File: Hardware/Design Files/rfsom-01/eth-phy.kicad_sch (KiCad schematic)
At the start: 1 part, among them U6 KSZ9131RNXI-TR

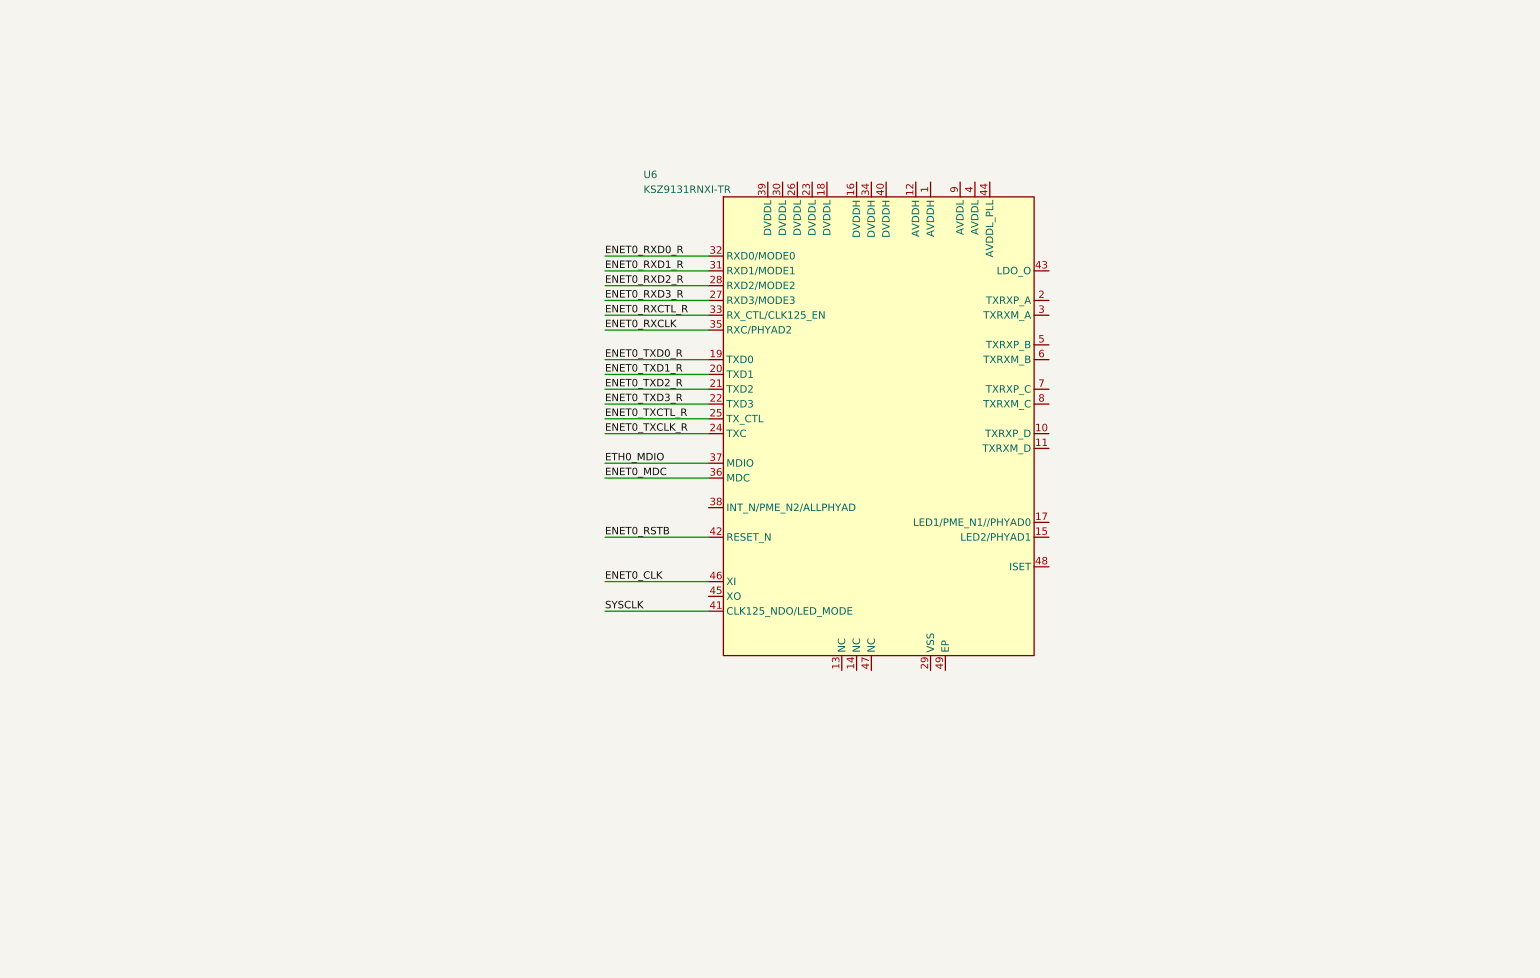
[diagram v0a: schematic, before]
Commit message: ps progress; added ftdi; mezz pinout pedinging;
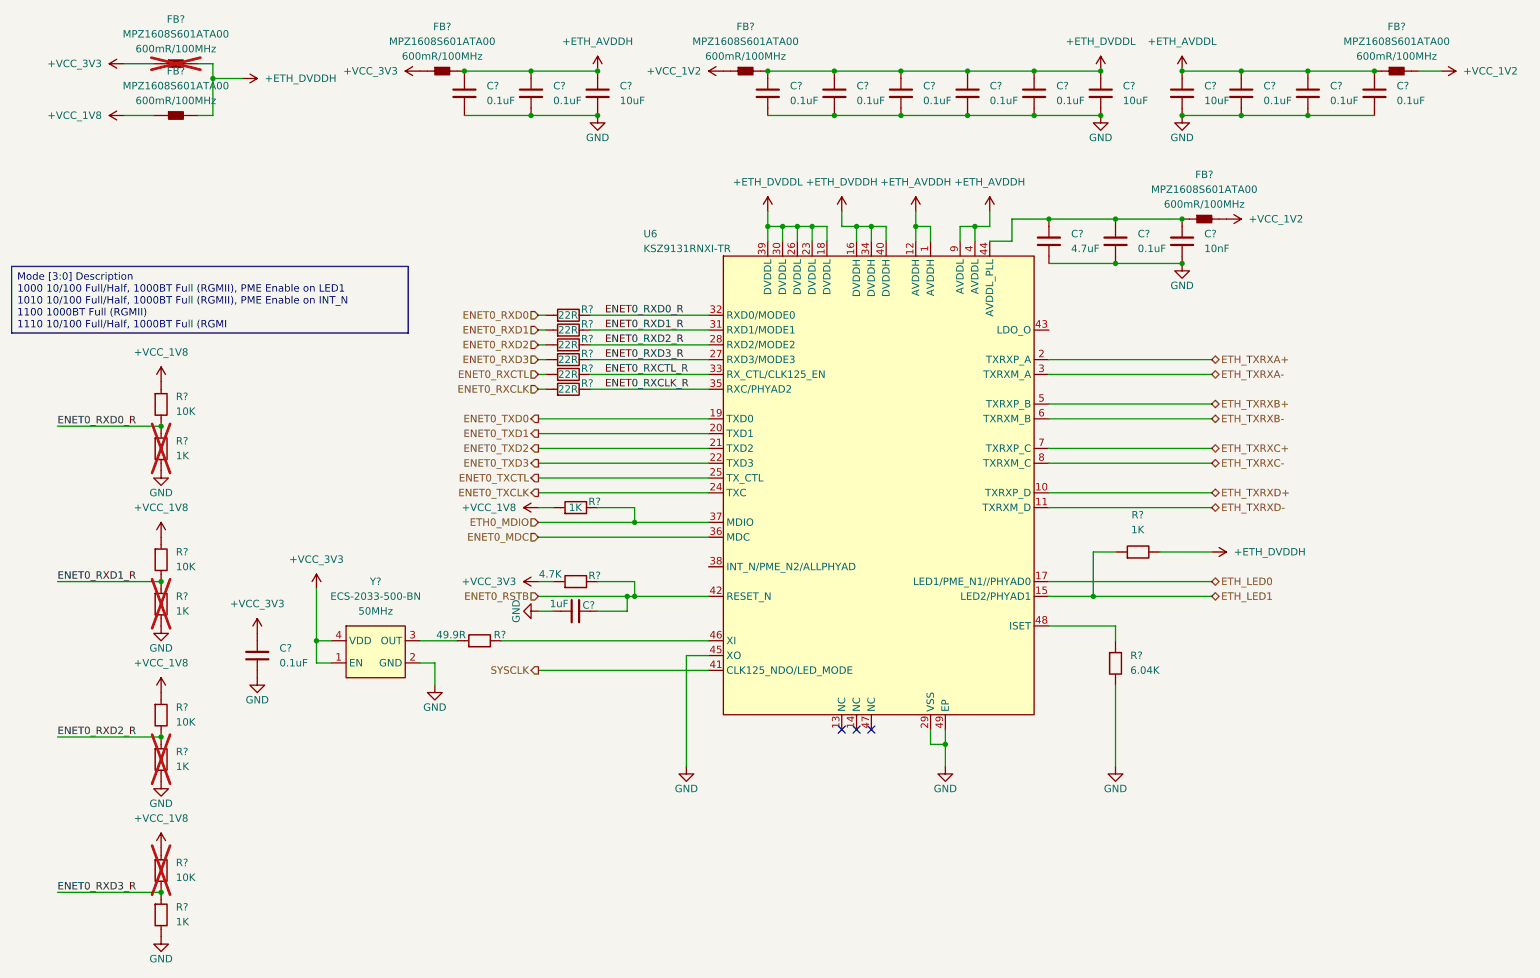
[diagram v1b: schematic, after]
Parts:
- added C? (x12): CL05B104KA5NNNC, Capacitor_SMD:C_0402_1005Metric_Pad0.74x0.62mm_HandSolder, symbol Capacitors:CL05B104KA5NNNC
- added C? (x3): CL31A106KBHNNNE, Capacitor_SMD:C_1206_3216Metric_Pad1.33x1.80mm_HandSolder, symbol Capacitors:CL31A106KBHNNNE
- added C?: CL10B105KA8NNNC, Capacitor_SMD:C_0603_1608Metric_Pad1.08x0.95mm_HandSolder, symbol Capacitors:CL10B105KA8NNNC
- added C?: CL05B103KB5NNNC, Capacitor_SMD:C_0402_1005Metric, symbol Capacitors:CL05B103KB5NNNC
- added C?: CL21B475KAFNNNE, Capacitor_SMD:C_0805_2012Metric_Pad1.18x1.45mm_HandSolder, symbol Capacitors:CL21B475KAFNNNE
- added FB? (x6): MPZ1608S601ATA00, Resistor_SMD:R_0603_1608Metric, symbol Inductors:MPZ1608S601ATA00
- added R? (x6): RC0402FR-0722RL, Resistor_SMD:R_0402_1005Metric, symbol Resistors:RC0402FR-0722RL
- added R? (x6): RC0603FR-071KL, Resistor_SMD:R_0603_1608Metric_Pad0.98x0.95mm_HandSolder, symbol Resistors:RC0603FR-071KL
- added R? (x4): RC0603FR-0710KL, Resistor_SMD:R_0603_1608Metric_Pad0.98x0.95mm_HandSolder, symbol Resistors:RC0603FR-0710KL
- added R?: RC0603FR-076K04L, Resistor_SMD:R_0603_1608Metric, symbol Resistors:RC0603FR-076K04L
- added R?: RES_01, Resistor_SMD:R_0402_1005Metric, symbol Resistors:RC0402FR-074K7L
- added R?: RC0603FR-0749R9L, Resistor_SMD:R_0603_1608Metric, symbol Resistors:RC0603FR-0749R9L
- added Y?: ECS-2033-500-BN, Miscellaneous:ECS-2033-500-BN, symbol Miscellaneous:ECS-2033-500-BN
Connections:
- net ENET0_RSTB: now also C?.2, R?.2
- net ENET0_RXCLK: now also R?.1; no longer U6.35 (RXC/PHYAD2)
- net ENET0_RXCTL_R: now also R?.2
- net ENET0_RXD0_R: now also R?.1, R?.2, R?.2
- net ENET0_RXD1_R: now also R?.1, R?.2, R?.2
- net ENET0_RXD2_R: now also R?.1, R?.2, R?.2
- net ENET0_RXD3_R: now also R?.1, R?.2, R?.2
- net ETH0_MDIO: now also R?.2
- net +ETH_AVDDH: now reaches U6.1 (AVDDH)
- net +ETH_AVDDH: now also U6.12 (AVDDH), U6.4 (AVDDL), U6.9 (AVDDL), C?.1, C?.1, C?.1, FB?.2
- net ETH_TXRXD+: now reaches U6.10 (TXRXP_D)
- net ETH_TXRXD-: now reaches U6.11 (TXRXM_D)
- net ETH_LED1: now reaches U6.15 (LED2/PHYAD1)
- net ETH_LED1: now also R?.1
- net +ETH_DVDDH: now reaches U6.16 (DVDDH)
- net +ETH_DVDDH: now also U6.34 (DVDDH), U6.40 (DVDDH), FB?.2, FB?.2, R?.2
- net ETH_LED0: now reaches U6.17 (LED1/PME_N1//PHYAD0)
- net +ETH_DVDDL: now reaches U6.18 (DVDDL)
- net +ETH_DVDDL: now also U6.23 (DVDDL), U6.26 (DVDDL), U6.30 (DVDDL), U6.39 (DVDDL), C?.1, C?.1, C?.1, C?.1, C?.1, C?.1, FB?.2
- net ETH_TXRXA+: now reaches U6.2 (TXRXP_A)
- net GND: now reaches U6.29 (VSS)
- net GND: now also U6.45 (XO), U6.49 (EP), C?.1, C?.2, C?.2, C?.2, C?.2, C?.2, C?.2, C?.2, C?.2, C?.2, C?.2, C?.2, C?.2, C?.2, C?.2, C?.2, C?.2, C?.2, R?.2, R?.2, R?.2, R?.2, R?.2, Y?.2 (GND)
- net ETH_TXRXA-: now reaches U6.3 (TXRXM_A)
- net at U6.44 (AVDDL_PLL): now also C?.1, C?.1, C?.1, FB?.1
- net at U6.48 (ISET): now also R?.1
- net ETH_TXRXB+: now reaches U6.5 (TXRXP_B)
- net ETH_TXRXB-: now reaches U6.6 (TXRXM_B)
- net ETH_TXRXC+: now reaches U6.7 (TXRXP_C)
- net ETH_TXRXC-: now reaches U6.8 (TXRXM_C)
- net ENET0_CLK: no longer names the net of U6.46 (XI)
- net ENET0_CLK: now also R?.2
- net ENET0_TXCLK_R renamed ENET0_TXCLK
- net ENET0_TXCTL_R renamed ENET0_TXCTL
- net ENET0_TXD0_R renamed ENET0_TXD0
- net ENET0_TXD1_R renamed ENET0_TXD1
- net ENET0_TXD2_R renamed ENET0_TXD2
- net ENET0_TXD3_R renamed ENET0_TXD3
- new net: R?.1, Y?.3 (OUT)
- new net +ETH_AVDDL: C?.1, C?.1, C?.1, C?.1, FB?.1
- new net +VCC_1V2: FB?.1, FB?.2, FB?.2
- new net +VCC_1V8: FB?.1, R?.1, R?.1, R?.1, R?.1, R?.1
- new net +VCC_3V3: C?.1, FB?.1, FB?.1, R?.1, Y?.1 (EN), Y?.4 (VDD)
- new net ENET0_RXCLK_R: R?.2, U6.35 (RXC/PHYAD2)
- new net ENET0_RXCTL: R?.1
- new net ENET0_RXD0: R?.1
- new net ENET0_RXD1: R?.1
- new net ENET0_RXD2: R?.1
- new net ENET0_RXD3: R?.1
- no-connect marks 0 -> 3
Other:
- moved on the sheet: U6
